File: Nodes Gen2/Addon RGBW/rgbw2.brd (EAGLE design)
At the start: 77.1 x 48 mm, 33 parts, among them Q1 BUZ11SD, Q2 BUZ11SD, Q3 BUZ11SD, Q4 BUZ11SD, Q5 BUZ11SD, Q6 BUZ11SD, Q7 BUZ11SD, Q8 BUZ11SD

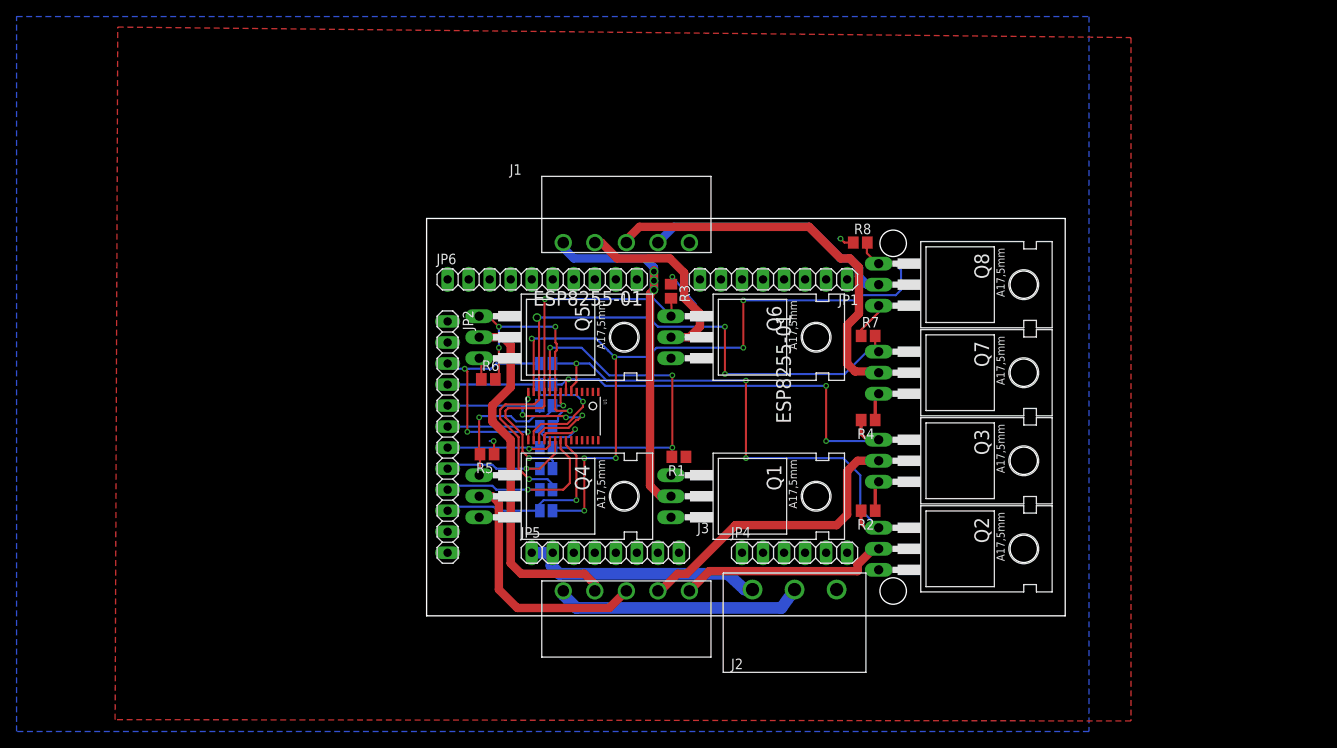
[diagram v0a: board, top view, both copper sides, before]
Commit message: gen 2 dev + bom
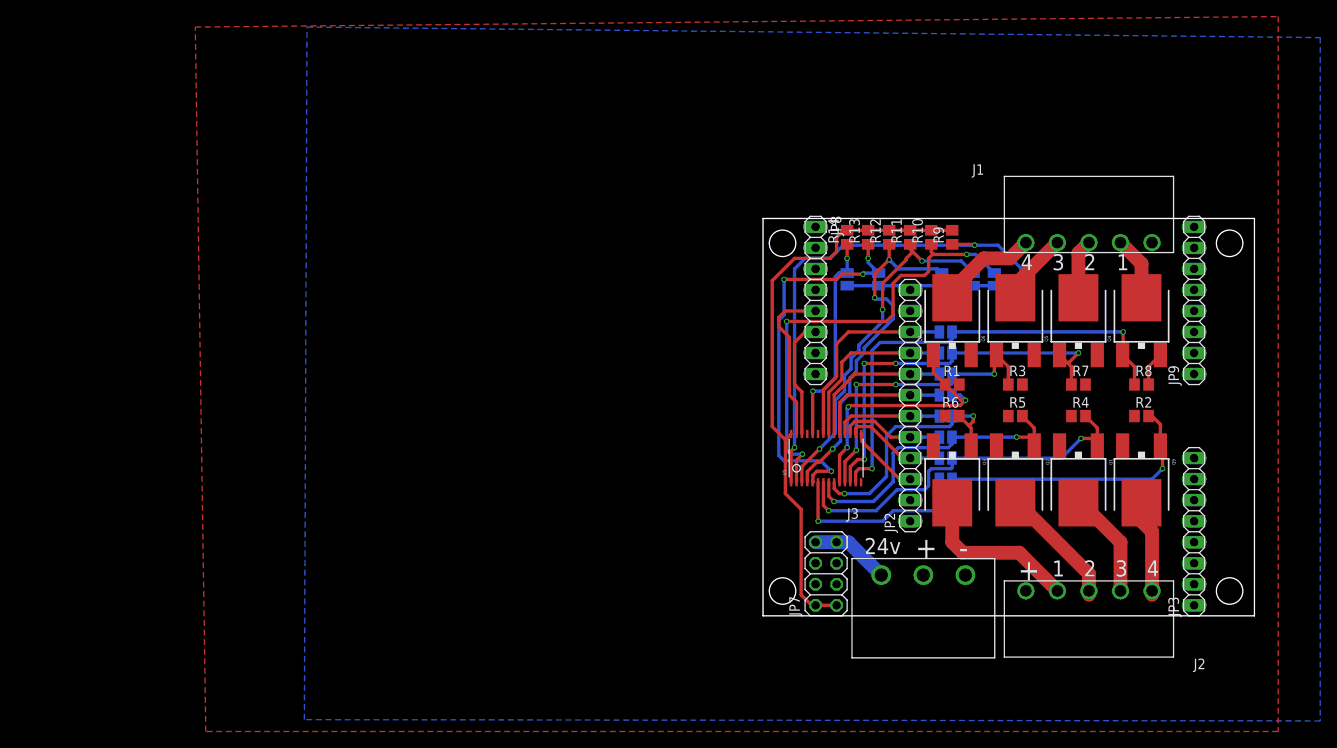
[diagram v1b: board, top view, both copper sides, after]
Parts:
- removed JP1, JP5: (no value), pinhead:1X08
- removed JP4: (no value), pinhead:1X06
- removed JP6: (no value), pinhead:1X10
- removed Q8: BUZ11SD, transistor-fet:TO220
- added JP3, JP8, JP9: (no value), pinhead:1X08
- added JP7: (no value), pinhead:2X04
- added Q9: MOSFET-NCHANNELFDD8780, SparkFun-DiscreteSemi:DPAK
- added R10, R11, R12, R13, R14, R9: (no value), schlager_passiv:R0805
- added SJ10, SJ11, SJ12, SJ13, SJ14, SJ6: (no value), jumper:SJ
- Q1, Q2, Q3, Q4, Q5, Q6, Q7: value BUZ11SD -> MOSFET-NCHANNELFDD8780; device transistor-fet:TO220 -> SparkFun-DiscreteSemi:DPAK
- moved Q4 77.0 mm to (86.4, 36.8), turned to 0 degrees
- moved Q5 66.1 mm to (78.7, 36.8), turned to 0 degrees
- moved R5 64.0 mm to (71.1, 24.1), turned to 0 degrees
- moved R6 56.2 mm to (63.5, 24.1)
- moved JP2 56.0 mm to (58.4, 25.4), turned to 90 degrees
- moved J1 55.9 mm to (76.2, 45.1)
- moved J2 55.9 mm to (83.8, 3.02)
- moved SJ9 52.9 mm to (62.7, 34.3)
- moved SJ7 51.0 mm to (62.7, 31.8)
- moved SJ1 50.2 mm to (62.7, 16.5)
- moved SJ8 49.6 mm to (62.7, 29.2)
- moved SJ2 49.1 mm to (62.7, 19.1)
- moved SJ5 48.7 mm to (62.7, 26.7)
- moved SJ3 48.4 mm to (62.7, 21.6)
- moved SJ4 48.3 mm to (62.7, 24.1)
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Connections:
- removed net A3_SCL2: JP4.4
- removed net A4_SDA2: JP4.5
- removed net A5: JP4.6
- removed net AREF: JP6.8
- removed net VDD: U1.28
- new net A3_V24: JP8.4
- new net N$1: R9.1, SJ6.2, U1.1
- new net N$10: R10.1, SJ10.2, U1.2
- new net N$11: R11.1, SJ11.2, U1.3
- new net N$12: R12.1, SJ12.2, U1.4
- new net N$13: R13.1, SJ13.2, U1.5
- new net N$14: R14.1, SJ14.2, U1.24
- new net RESERVE: JP9.7
- new net RESERVE2: JP9.8
- net A0: now also JP8.1; no longer JP4.1
- net A1: now also JP8.2; no longer JP4.2
- net A2: now also JP8.3; no longer JP4.3
- net A4_SDA: now also JP8.5, U1.27; no longer JP6.9
- net A5_SCL: now also JP8.6, U1.26; no longer JP6.10
- net A6: now also JP8.7; no longer JP5.8
- net A7: now also JP8.8; no longer JP5.7
- net D10_SS: now also JP9.3; no longer JP6.3
- net D11_MOSI: now also JP9.4; no longer JP6.4
- net D12_MISO: now also JP9.5; no longer JP6.5
- net D13_SCK: now also JP9.6; no longer JP6.6
- net D2: now also JP3.3; no longer JP1.3
- net D3: now also JP3.4; no longer JP1.4
- net D4: now also JP3.5; no longer JP1.5
- net D5: now also JP3.6; no longer JP1.6
- net D6: now also JP3.7; no longer JP1.7
- net D7: now also JP3.8; no longer JP1.8
- net D8: now also JP9.1; no longer JP6.1
- net D9: now also JP9.2; no longer JP6.2
- net GND: now also JP7.3, JP7.4, Q9.3, SJ10.1, SJ11.1, SJ12.1, SJ13.1, SJ14.1, SJ6.1; no longer JP5.3, JP5.4, JP6.7, Q8.3
- net LED0: now also Q9.1; no longer Q2.1
- net LED1: now also Q1.1; no longer Q3.1
- net LED2: now also Q2.1; no longer Q4.1
- net LED3: now also Q3.1; no longer Q5.1
- net LED4: now also Q7.1; no longer Q1.1
- net LED6: now also Q5.1; no longer Q7.1
- net LED7: now also Q4.1; no longer Q8.1
- net N$2: now also Q9.4; no longer Q2.2
- net N$3: now also Q1.4; no longer Q3.2
- net N$4: now also Q5.4; no longer Q7.2
- net N$5: now also Q2.4; no longer Q4.2
- net N$6: now also Q3.4; no longer Q5.2
- net N$7: now also Q4.4; no longer Q8.2
- net N$8: now also Q7.4; no longer Q1.2
- net N$9: now also Q6.4; no longer Q6.2
- net P24P: now also JP7.7, JP7.8; no longer JP5.1, JP5.2
- net P24X: now also JP7.5, JP7.6
- net P5V: now also JP7.1, JP7.2, R10.2, R11.2, R12.2, R13.2, R14.2, R9.2, U1.28; no longer JP5.5, JP5.6
- net RX: now also JP3.1; no longer JP1.1
- net TX: now also JP3.2; no longer JP1.2
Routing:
- net P5V: track 0.00 -> 70.5 mm
- net N$1: track 0.00 -> 59.2 mm, vias 0 -> 2
- net N$10: track 0.00 -> 55.2 mm, vias 0 -> 3
- net N$13: track 0.00 -> 47.7 mm, vias 0 -> 4
- net N$12: track 0.00 -> 43.2 mm, vias 0 -> 3
- net N$11: track 0.00 -> 42.8 mm, vias 0 -> 3
- net N$4: track 47.6 -> 7.19 mm
- net LED7: track 93.7 -> 56.4 mm, vias 7 -> 2
- net N$8: track 44.6 -> 12.2 mm, vias 3 -> 0
- net LED6: track 79.9 -> 48.5 mm
- net P24X: track 30.2 -> 0.00 mm
- net N$14: track 0.00 -> 25.9 mm, vias 0 -> 2
- net N$6: track 44.4 -> 19.9 mm
- net N$3: track 36.2 -> 12.9 mm
- net N$7: track 31.0 -> 7.72 mm
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- added copper zone on layer 1, net GND
- added copper zone on layer 16, net P24X
- removed copper zone on layer 16, net GND
- removed copper zone on layer 1, net P24X
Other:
- board size 77.1 x 48 mm -> 59.4 x 48 mm
- board text added: "+"
- board text added: "-"
- board text added: "1"
- board text added: "2"
- board text added: "24v"
- board text added: "3"
- board text added: "4"
- board text removed: "ESP8255-01"
- board text removed: "i2c"

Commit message: so much...
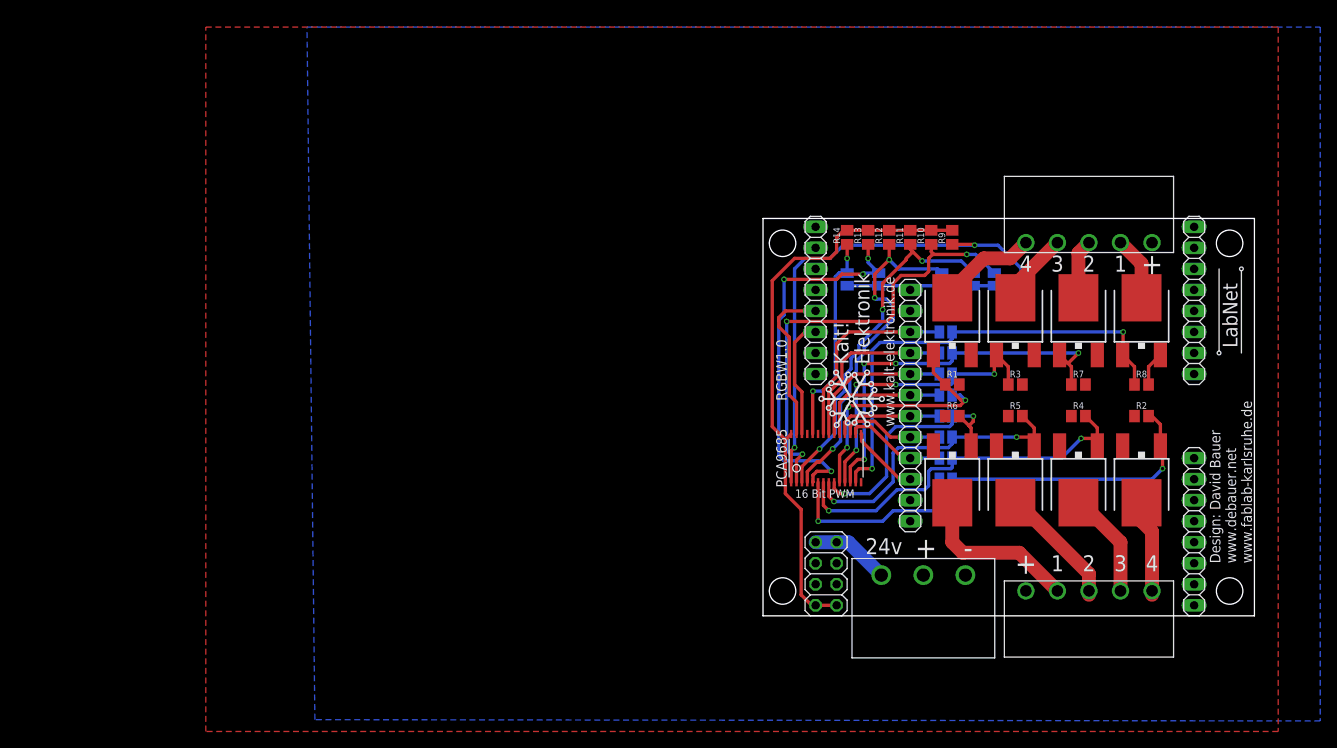
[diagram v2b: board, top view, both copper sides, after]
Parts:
- added U$1: (no value), debauer_special:KALT!ELEKTRONIK
- added U$2: (no value), debauer_special:LABNET
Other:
- board text added: "16 Bit PWM"
- board text added: "Design: David Bauer"
- board text added: "PCA9685"
- board text added: "RGBW1.0"
- board text added: "www.debauer.net"
- board text added: "www.fablab-karlsruhe.de"
- board text added: "www.kalt-elektronik.de"
